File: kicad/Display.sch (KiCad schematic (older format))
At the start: 34 parts, among them P201 CONN_01X06, P202 CONN_01X07, P203 CONN_01X06, P204 CONN_01X07, Q201 BC856BS, Q202 BC856BS, Q203 BC856BS, U201 SN74LS138, U202 74HC4511

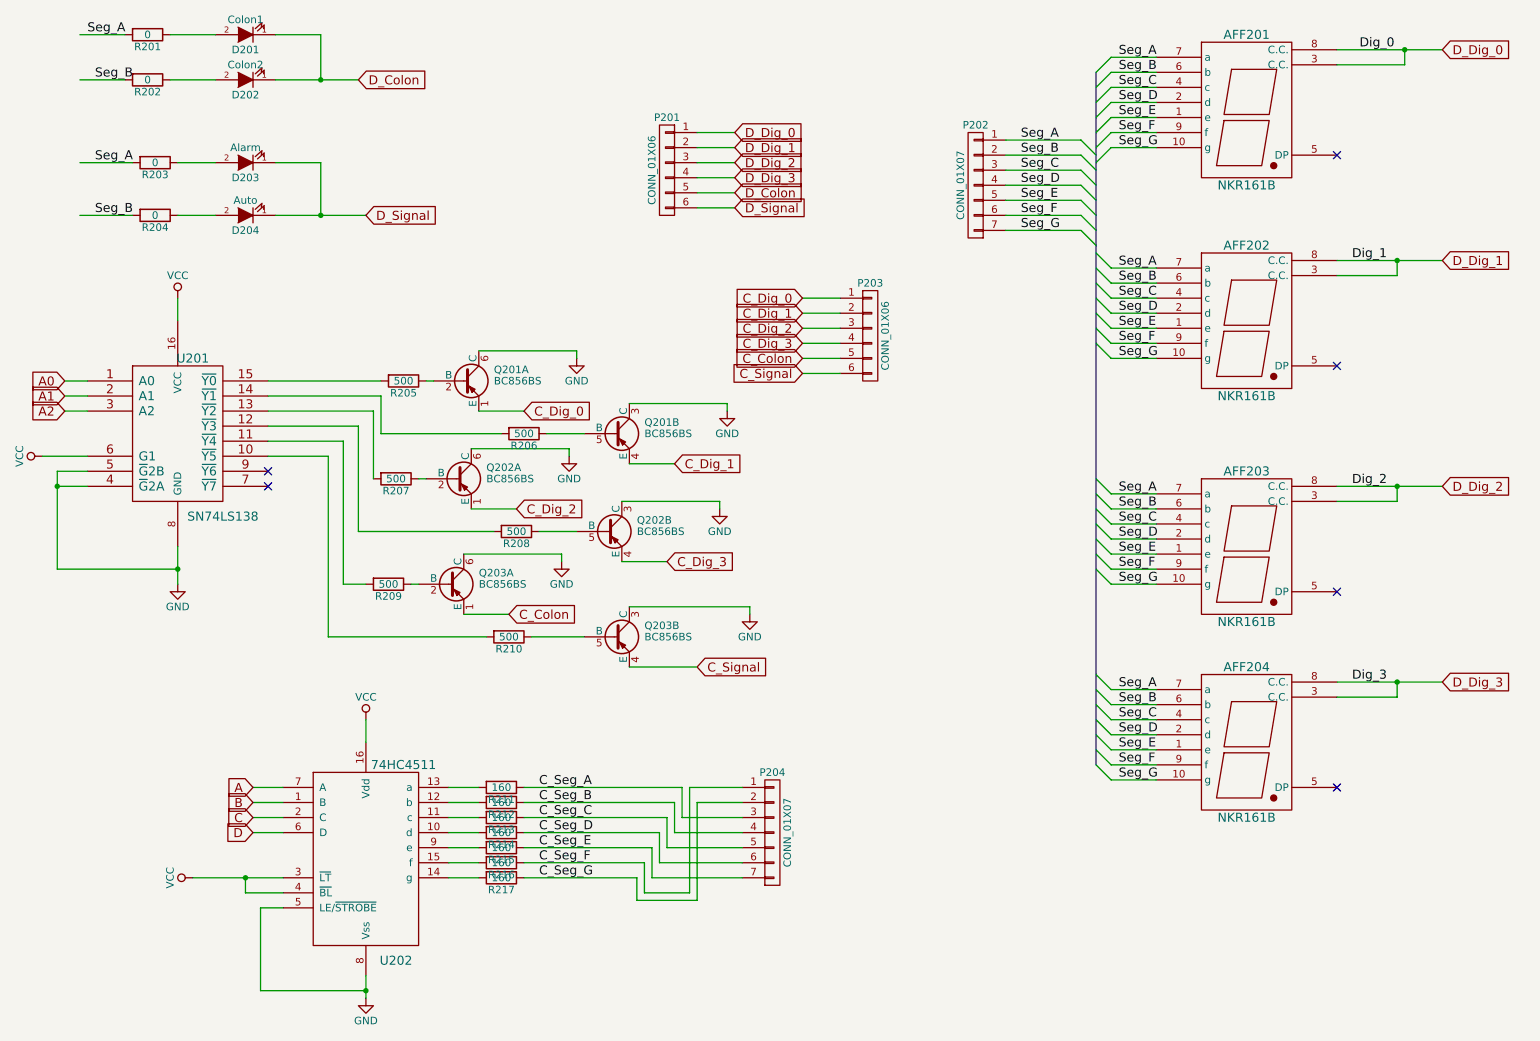
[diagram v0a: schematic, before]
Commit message: Changes to the gerbers
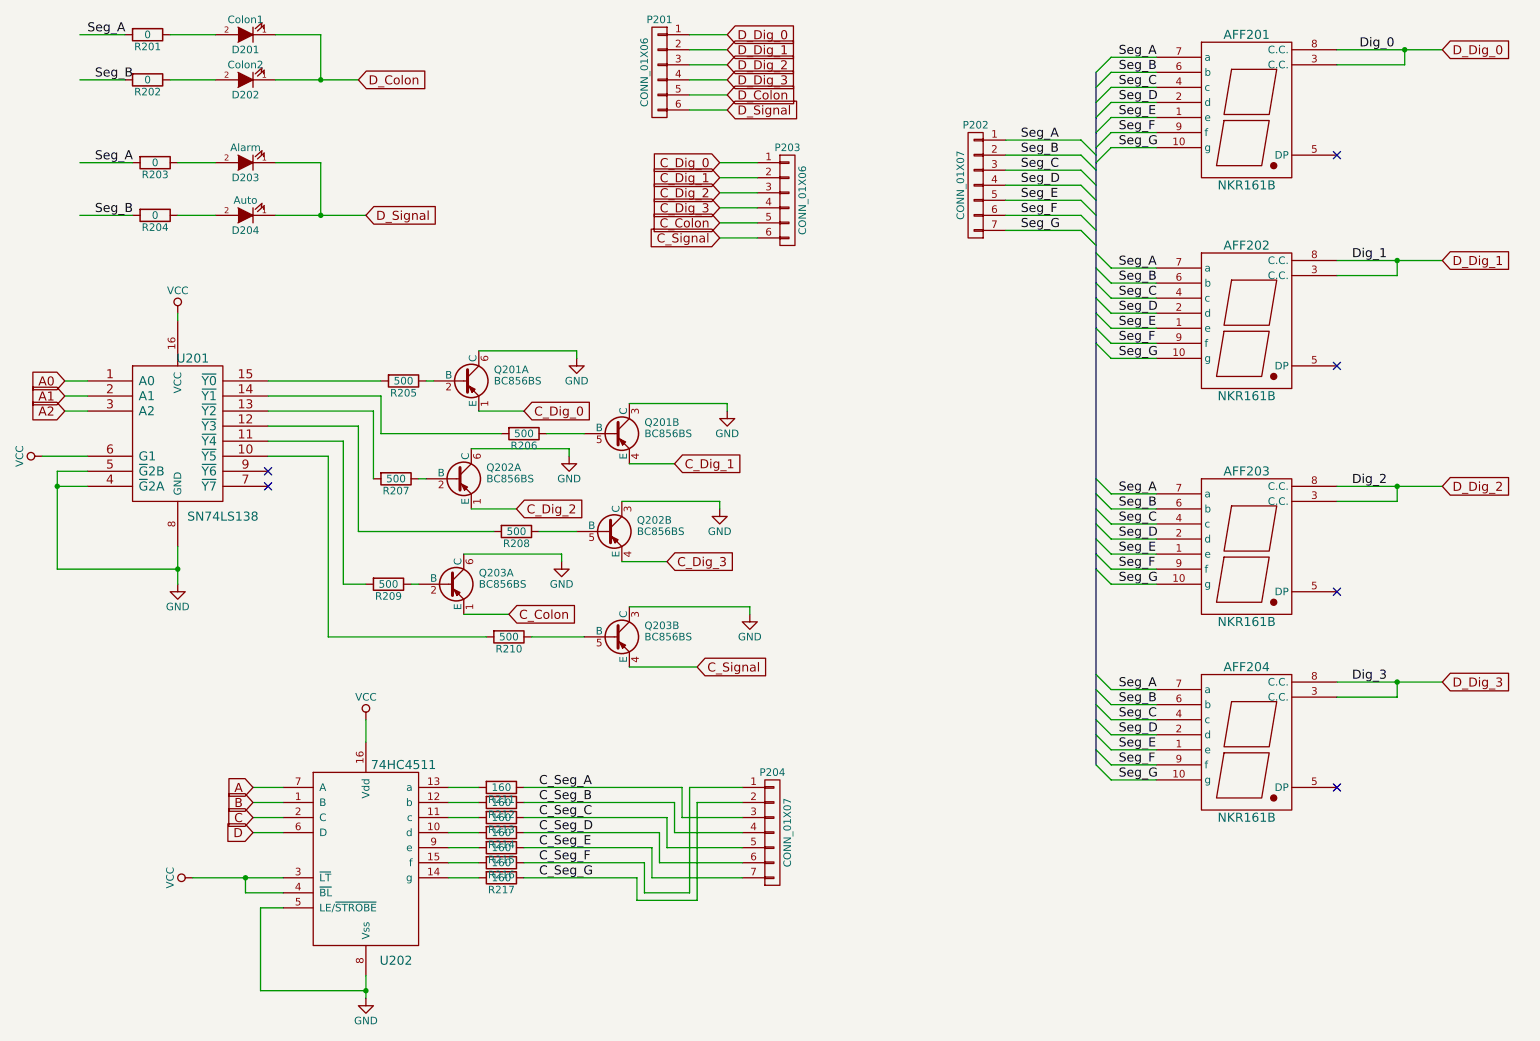
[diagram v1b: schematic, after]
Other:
- moved on the sheet: P201, P203
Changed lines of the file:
@@
 	9450 5150 9850 5150
 Wire Wire Line
-	9450 850  10150 850
+	9450 850  9900 850
+Wire Wire Line
+	9900 850  10150 850
 Wire Wire Line
 	9900 950  9900 850
@@
 	7250 2050 7750 2050
 Wire Wire Line
-	9450 2250 10150 2250
+	9450 2250 9850 2250
+Wire Wire Line
+	9850 2250 10150 2250
 Wire Wire Line
 	9450 950  9900 950
 Wire Wire Line
-	9450 3750 10150 3750
-Wire Wire Line
-	9450 5050 10150 5050
-Wire Bus Line
-	7850 1000 7850 5600
+	9450 3750 9850 3750
+Wire Wire Line
+	9850 3750 10150 3750
+Wire Wire Line
+	9450 5050 9850 5050
+Wire Wire Line
+	9850 5050 10150 5050
+Wire Bus Line
+	7850 1000 7850 1100
+Wire Bus Line
+	7850 1100 7850 1200
+Wire Bus Line
+	7850 1200 7850 1300
+Wire Bus Line
+	7850 1300 7850 1400
+Wire Bus Line
+	7850 1400 7850 1500
+Wire Bus Line
+	7850 1500 7850 1550
+Wire Bus Line
+	7850 1550 7850 1600
+Wire Bus Line
+	7850 1600 7850 1650
+Wire Bus Line
+	7850 1650 7850 1750
+Wire Bus Line
+	7850 1750 7850 1850
+Wire Bus Line
+	7850 1850 7850 1950
+Wire Bus Line
+	7850 1950 7850 2050
+Wire Bus Line
+	7850 2050 7850 2150
+Wire Bus Line
+	7850 2150 7850 2200
+Wire Bus Line
+	7850 2200 7850 2300
+Wire Bus Line
+	7850 2300 7850 2400
+Wire Bus Line
+	7850 2400 7850 2500
+Wire Bus Line
+	7850 2500 7850 2600
+Wire Bus Line
+	7850 2600 7850 2700
+Wire Bus Line
+	7850 2700 7850 2800
+Wire Bus Line
+	7850 2800 7850 3700
+Wire Bus Line
+	7850 3700 7850 3800
+Wire Bus Line
+	7850 3800 7850 3900
+Wire Bus Line
+	7850 3900 7850 4000
+Wire Bus Line
+	7850 4000 7850 4100
+Wire Bus Line
+	7850 4100 7850 4200
+Wire Bus Line
+	7850 4200 7850 4300
+Wire Bus Line
+	7850 4300 7850 5000
+Wire Bus Line
+	7850 5000 7850 5100
+Wire Bus Line
+	7850 5100 7850 5200
+Wire Bus Line
+	7850 5200 7850 5300
+Wire Bus Line
+	7850 5300 7850 5400
+Wire Bus Line
+	7850 5400 7850 5500
+Wire Bus Line
+	7850 5500 7850 5600
 $Comp
 L 74HC4511 U202
@@
 	2400 750  2700 750
 Wire Wire Line
-	2400 1950 3000 1950
-Wire Wire Line
-	2400 1050 2950 1050
+	2400 1950 2700 1950
+Wire Wire Line
+	2700 1950 3000 1950
+Wire Wire Line
+	2400 1050 2700 1050
+Wire Wire Line
+	2700 1050 2950 1050
 Connection ~ 2700 1050
 Wire Wire Line
@@
 L VCC #PWR015
 U 1 1 55871329
-P 1750 2500
-F 0 "#PWR015" H 1750 2350 50  0001 C CNN
-F 1 "VCC" H 1750 2650 50  0000 C CNN
-F 2 "" H 1750 2500 60  0000 C CNN
-F 3 "" H 1750 2500 60  0000 C CNN
-	1    1750 2500
-	1    0    0    -1
-$EndComp
-Wire Wire Line
-	1750 2500 1750 2650
+P 1750 2600
+F 0 "#PWR015" H 1750 2450 50  0001 C CNN
+F 1 "VCC" H 1750 2750 50  0000 C CNN
+F 2 "" H 1750 2600 60  0000 C CNN
+F 3 "" H 1750 2600 60  0000 C CNN
+	1    1750 2600
+	1    0    0    -1
+$EndComp
+Wire Wire Line
+	1750 2600 1750 2650
 $Comp
 L GND #PWR016
@@
 $EndComp
 Wire Wire Line
-	1750 4150 1750 4400
+	1750 4150 1750 4300
+Wire Wire Line
+	1750 4300 1750 4400
 Wire Wire Line
 	1150 3650 950  3650
 Wire Wire Line
-	950  3650 950  4300
+	950  3650 950  3750
+Wire Wire Line
+	950  3750 950  4300
 Wire Wire Line
 	950  4300 1750 4300
@@
 $EndComp
 Wire Wire Line
-	1850 6350 2450 6350
+	1850 6350 2200 6350
+Wire Wire Line
+	2200 6350 2450 6350
 Wire Wire Line
 	2450 6450 2200 6450
@@
 $EndComp
 Wire Wire Line
-	3000 7000 3000 7150
+	3000 7000 3000 7100
+Wire Wire Line
+	3000 7100 3000 7150
 Wire Wire Line
 	2450 6550 2300 6550
@@
 L CONN_01X06 P201
 U 1 1 5589B385
-P 5000 1650
-F 0 "P201" H 5000 2000 50  0000 C CNN
-F 1 "CONN_01X06" V 5100 1650 50  0000 C CNN
-F 2 "Pin_Headers:Pin_Header_Straight_1x06" H 5000 1650 60  0001 C CNN
-F 3 "" H 5000 1650 60  0000 C CNN
-	1    5000 1650
+P 4950 1000
+F 0 "P201" H 4950 1350 50  0000 C CNN
+F 1 "CONN_01X06" V 5050 1000 50  0000 C CNN
+F 2 "Pin_Headers:Pin_Header_Straight_1x06" H 4950 1000 60  0001 C CNN
+F 3 "" H 4950 1000 60  0000 C CNN
+	1    4950 1000
 	-1   0    0    -1
 $EndComp
-Text GLabel 5450 1400 2    60   Input ~ 0
+Text GLabel 5400 750  2    60   Input ~ 0
 D_Dig_0
-Text GLabel 5450 1500 2    60   Input ~ 0
+Text GLabel 5400 850  2    60   Input ~ 0
 D_Dig_1
-Text GLabel 5450 1600 2    60   Input ~ 0
+Text GLabel 5400 950  2    60   Input ~ 0
 D_Dig_2
-Text GLabel 5450 1700 2    60   Input ~ 0
+Text GLabel 5400 1050 2    60   Input ~ 0
 D_Dig_3
-Text GLabel 5450 1900 2    60   Input ~ 0
+Text GLabel 5400 1250 2    60   Input ~ 0
 D_Signal
-Text GLabel 5450 1800 2    60   Input ~ 0
+Text GLabel 5400 1150 2    60   Input ~ 0
 D_Colon
 Wire Wire Line
-	5200 1400 5450 1400
-Wire Wire Line
-	5450 1500 5200 1500
-Wire Wire Line
-	5200 1600 5450 1600
-Wire Wire Line
-	5450 1700 5200 1700
-Wire Wire Line
-	5200 1800 5450 1800
-Wire Wire Line
-	5450 1900 5200 1900
+	5150 750  5400 750
+Wire Wire Line
+	5400 850  5150 850
+Wire Wire Line
+	5150 950  5400 950
+Wire Wire Line
+	5400 1050 5150 1050
+Wire Wire Line
+	5150 1150 5400 1150
+Wire Wire Line
+	5400 1250 5150 1250
 $Comp
 L CONN_01X07 P204
@@
 L CONN_01X06 P203
 U 1 1 5589E43E
-P 6350 2750
-F 0 "P203" H 6350 3100 50  0000 C CNN
-F 1 "CONN_01X06" V 6450 2750 50  0000 C CNN
-F 2 "Pin_Headers:Pin_Header_Straight_1x06" H 6350 2750 60  0001 C CNN
-F 3 "" H 6350 2750 60  0000 C CNN
-	1    6350 2750
-	1    0    0    -1
-$EndComp
-Text GLabel 5900 2500 0    60   Input ~ 0
+P 5800 1850
+F 0 "P203" H 5800 2200 50  0000 C CNN
+F 1 "CONN_01X06" V 5900 1850 50  0000 C CNN
+F 2 "Pin_Headers:Pin_Header_Straight_1x06" H 5800 1850 60  0001 C CNN
+F 3 "" H 5800 1850 60  0000 C CNN
+	1    5800 1850
+	1    0    0    -1
+$EndComp
+Text GLabel 5350 1600 0    60   Input ~ 0
 C_Dig_0
-Text GLabel 5900 2600 0    60   Input ~ 0
+Text GLabel 5350 1700 0    60   Input ~ 0
 C_Dig_1
-Text GLabel 5900 2700 0    60   Input ~ 0
+Text GLabel 5350 1800 0    60   Input ~ 0
 C_Dig_2
-Text GLabel 5900 2800 0    60   Input ~ 0
+Text GLabel 5350 1900 0    60   Input ~ 0
 C_Dig_3
-Text GLabel 5900 2900 0    60   Input ~ 0
+Text GLabel 5350 2000 0    60   Input ~ 0
 C_Colon
-Text GLabel 5900 3000 0    60   Input ~ 0
+Text GLabel 5350 2100 0    60   Input ~ 0
 C_Signal
 Wire Wire Line
-	5900 2500 6150 2500
-Wire Wire Line
-	6150 2600 5900 2600
-Wire Wire Line
-	5900 2700 6150 2700
-Wire Wire Line
-	6150 2800 5900 2800
-Wire Wire Line
-	5900 2900 6150 2900
-Wire Wire Line
-	6150 3000 5900 3000
+	5350 1600 5600 1600
+Wire Wire Line
+	5600 1700 5350 1700
+Wire Wire Line
+	5350 1800 5600 1800
+Wire Wire Line
+	5600 1900 5350 1900
+Wire Wire Line
+	5350 2000 5600 2000
+Wire Wire Line
+	5600 2100 5350 2100
 $Comp
 L BC856BS Q201

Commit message: small correction
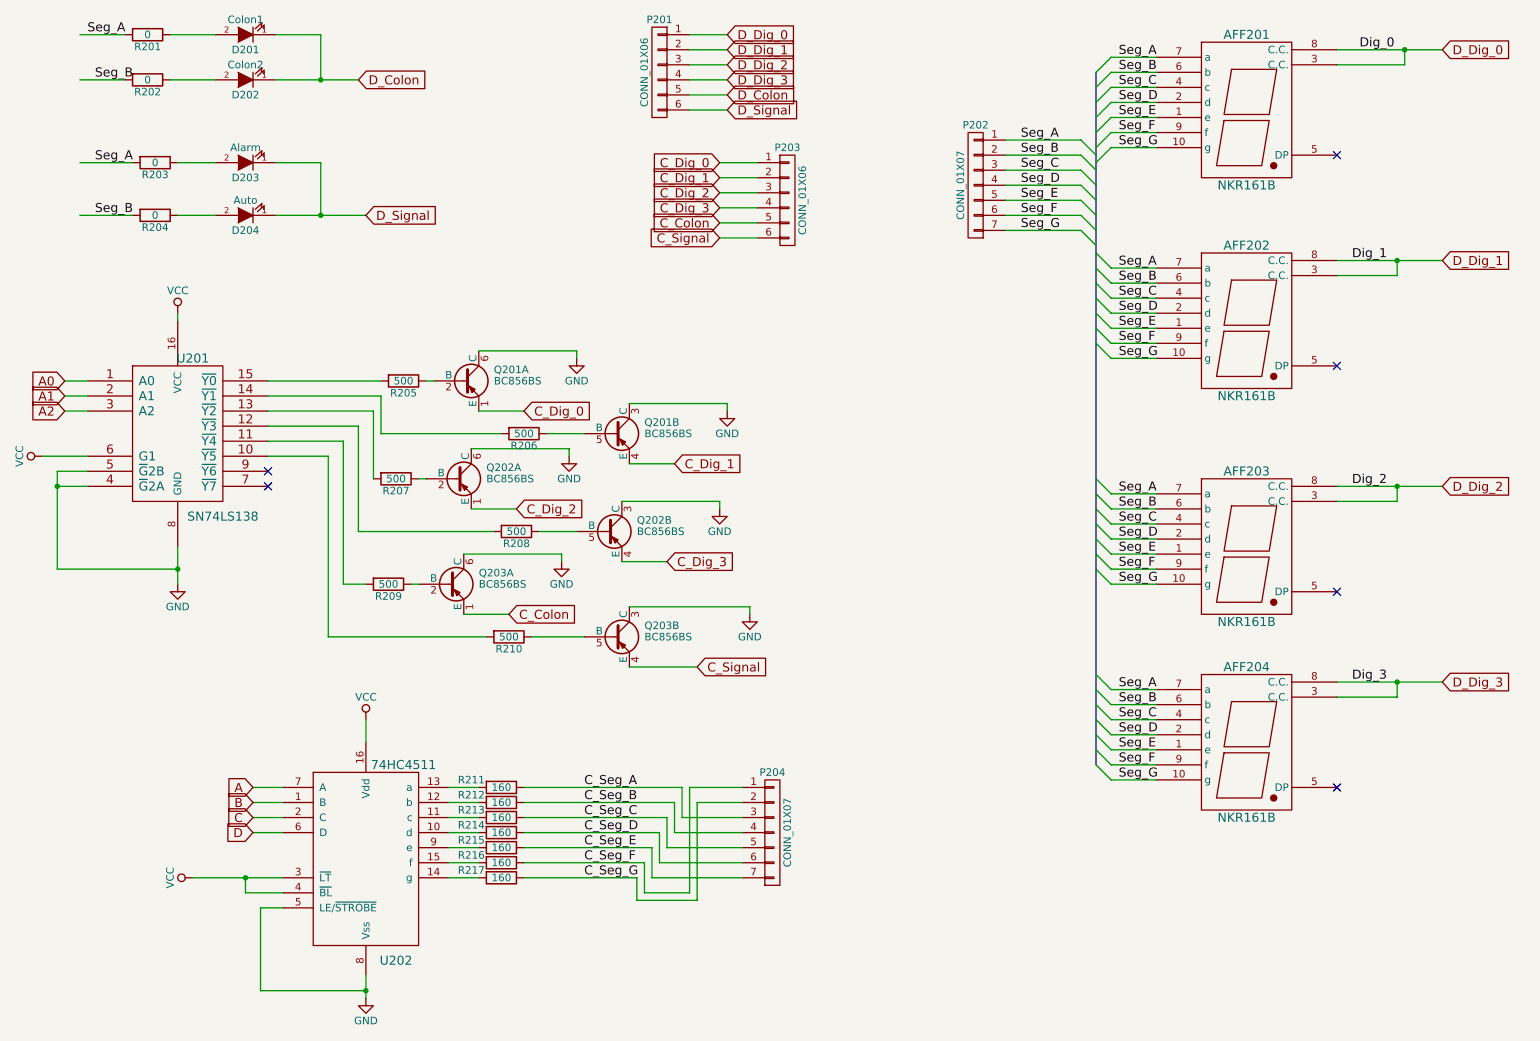
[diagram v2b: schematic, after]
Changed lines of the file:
@@
 	9450 5150 9850 5150
 Wire Wire Line
-	9450 850  9900 850
-Wire Wire Line
-	9900 850  10150 850
+	9450 850  10150 850
 Wire Wire Line
 	9900 950  9900 850
@@
 	7250 2050 7750 2050
 Wire Wire Line
-	9450 2250 9850 2250
-Wire Wire Line
-	9850 2250 10150 2250
+	9450 2250 10150 2250
 Wire Wire Line
 	9450 950  9900 950
 Wire Wire Line
-	9450 3750 9850 3750
-Wire Wire Line
-	9850 3750 10150 3750
-Wire Wire Line
-	9450 5050 9850 5050
-Wire Wire Line
-	9850 5050 10150 5050
+	9450 3750 10150 3750
+Wire Wire Line
+	9450 5050 10150 5050
 Wire Bus Line
-	7850 1000 7850 1100
-Wire Bus Line
-	7850 1100 7850 1200
-Wire Bus Line
-	7850 1200 7850 1300
-Wire Bus Line
-	7850 1300 7850 1400
-Wire Bus Line
-	7850 1400 7850 1500
-Wire Bus Line
-	7850 1500 7850 1550
-Wire Bus Line
-	7850 1550 7850 1600
-Wire Bus Line
-	7850 1600 7850 1650
-Wire Bus Line
-	7850 1650 7850 1750
-Wire Bus Line
-	7850 1750 7850 1850
-Wire Bus Line
-	7850 1850 7850 1950
-Wire Bus Line
-	7850 1950 7850 2050
-Wire Bus Line
-	7850 2050 7850 2150
-Wire Bus Line
-	7850 2150 7850 2200
-Wire Bus Line
-	7850 2200 7850 2300
-Wire Bus Line
-	7850 2300 7850 2400
-Wire Bus Line
-	7850 2400 7850 2500
-Wire Bus Line
-	7850 2500 7850 2600
-Wire Bus Line
-	7850 2600 7850 2700
-Wire Bus Line
-	7850 2700 7850 2800
-Wire Bus Line
-	7850 2800 7850 3700
-Wire Bus Line
-	7850 3700 7850 3800
-Wire Bus Line
-	7850 3800 7850 3900
-Wire Bus Line
-	7850 3900 7850 4000
-Wire Bus Line
-	7850 4000 7850 4100
-Wire Bus Line
-	7850 4100 7850 4200
-Wire Bus Line
-	7850 4200 7850 4300
-Wire Bus Line
-	7850 4300 7850 5000
-Wire Bus Line
-	7850 5000 7850 5100
-Wire Bus Line
-	7850 5100 7850 5200
-Wire Bus Line
-	7850 5200 7850 5300
-Wire Bus Line
-	7850 5300 7850 5400
-Wire Bus Line
-	7850 5400 7850 5500
-Wire Bus Line
-	7850 5500 7850 5600
+	7850 1000 7850 5600
 $Comp
 L 74HC4511 U202
@@
 	2400 750  2700 750
 Wire Wire Line
-	2400 1950 2700 1950
-Wire Wire Line
-	2700 1950 3000 1950
-Wire Wire Line
-	2400 1050 2700 1050
-Wire Wire Line
-	2700 1050 2950 1050
+	2400 1950 3000 1950
+Wire Wire Line
+	2400 1050 2950 1050
 Connection ~ 2700 1050
 Wire Wire Line
@@
 U 1 1 5587356B
 P 3900 5750
-F 0 "R211" V 3980 5750 50  0000 C CNN
+F 0 "R211" V 3850 5550 50  0000 C CNN
 F 1 "160" V 3900 5750 50  0000 C CNN
 F 2 "Resistors_SMD:R_0805_HandSoldering" V 3830 5750 30  0001 C CNN
@@
 U 1 1 55873774
 P 3900 5850
-F 0 "R212" V 3980 5850 50  0000 C CNN
+F 0 "R212" V 3850 5650 50  0000 C CNN
 F 1 "160" V 3900 5850 50  0000 C CNN
 F 2 "Resistors_SMD:R_0805_HandSoldering" V 3830 5850 30  0001 C CNN
@@
 U 1 1 5587381A
 P 3900 5950
-F 0 "R213" V 3980 5950 50  0000 C CNN
+F 0 "R213" V 3850 5750 50  0000 C CNN
 F 1 "160" V 3900 5950 50  0000 C CNN
 F 2 "Resistors_SMD:R_0805_HandSoldering" V 3830 5950 30  0001 C CNN
@@
 U 1 1 55873877
 P 3900 6050
-F 0 "R214" V 3980 6050 50  0000 C CNN
+F 0 "R214" V 3850 5850 50  0000 C CNN
 F 1 "160" V 3900 6050 50  0000 C CNN
 F 2 "Resistors_SMD:R_0805_HandSoldering" V 3830 6050 30  0001 C CNN
@@
 U 1 1 55873973
 P 3900 6150
-F 0 "R215" V 3980 6150 50  0000 C CNN
+F 0 "R215" V 3850 5950 50  0000 C CNN
 F 1 "160" V 3900 6150 50  0000 C CNN
 F 2 "Resistors_SMD:R_0805_HandSoldering" V 3830 6150 30  0001 C CNN
@@
 U 1 1 558739F1
 P 3900 6250
-F 0 "R216" V 3980 6250 50  0000 C CNN
+F 0 "R216" V 3850 6050 50  0000 C CNN
 F 1 "160" V 3900 6250 50  0000 C CNN
 F 2 "Resistors_SMD:R_0805_HandSoldering" V 3830 6250 30  0001 C CNN
@@
 U 1 1 55873A73
 P 3900 6350
-F 0 "R217" V 3980 6350 50  0000 C CNN
+F 0 "R217" V 3850 6150 50  0000 C CNN
 F 1 "160" V 3900 6350 50  0000 C CNN
 F 2 "Resistors_SMD:R_0805_HandSoldering" V 3830 6350 30  0001 C CNN
@@
 $EndComp
 Wire Wire Line
-	1750 4150 1750 4300
-Wire Wire Line
-	1750 4300 1750 4400
+	1750 4150 1750 4400
 Wire Wire Line
 	1150 3650 950  3650
 Wire Wire Line
-	950  3650 950  3750
-Wire Wire Line
-	950  3750 950  4300
+	950  3650 950  4300
 Wire Wire Line
 	950  4300 1750 4300
@@
 $EndComp
 Wire Wire Line
-	1850 6350 2200 6350
-Wire Wire Line
-	2200 6350 2450 6350
+	1850 6350 2450 6350
 Wire Wire Line
 	2450 6450 2200 6450
@@
 $EndComp
 Wire Wire Line
-	3000 7000 3000 7100
-Wire Wire Line
-	3000 7100 3000 7150
+	3000 7000 3000 7150
 Wire Wire Line
 	2450 6550 2300 6550
@@
 	1    0    0    -1
 $EndComp
-Text Label 4150 5750 0    60   ~ 0
+Text Label 4450 5750 0    60   ~ 0
 C_Seg_A
-Text Label 4150 5850 0    60   ~ 0
+Text Label 4450 5850 0    60   ~ 0
 C_Seg_B
-Text Label 4150 5950 0    60   ~ 0
+Text Label 4450 5950 0    60   ~ 0
 C_Seg_C
-Text Label 4150 6050 0    60   ~ 0
+Text Label 4450 6050 0    60   ~ 0
 C_Seg_D
-Text Label 4150 6150 0    60   ~ 0
+Text Label 4450 6150 0    60   ~ 0
 C_Seg_E
-Text Label 4150 6250 0    60   ~ 0
+Text Label 4450 6250 0    60   ~ 0
 C_Seg_F
-Text Label 4150 6350 0    60   ~ 0
+Text Label 4450 6350 0    60   ~ 0
 C_Seg_G
 Wire Wire Line
